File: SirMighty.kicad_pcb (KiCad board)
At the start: 2 copper layers, 61 x 20.5 mm, 49 parts, among them J1 Conn_01x20, J2 Conn_01x20, J3 USB_B_Micro, Q1 Q_DUAL_PMOS_S1G1D2S2G2D1, U2 AP7365-W-7, U4 AZ1117-5.0

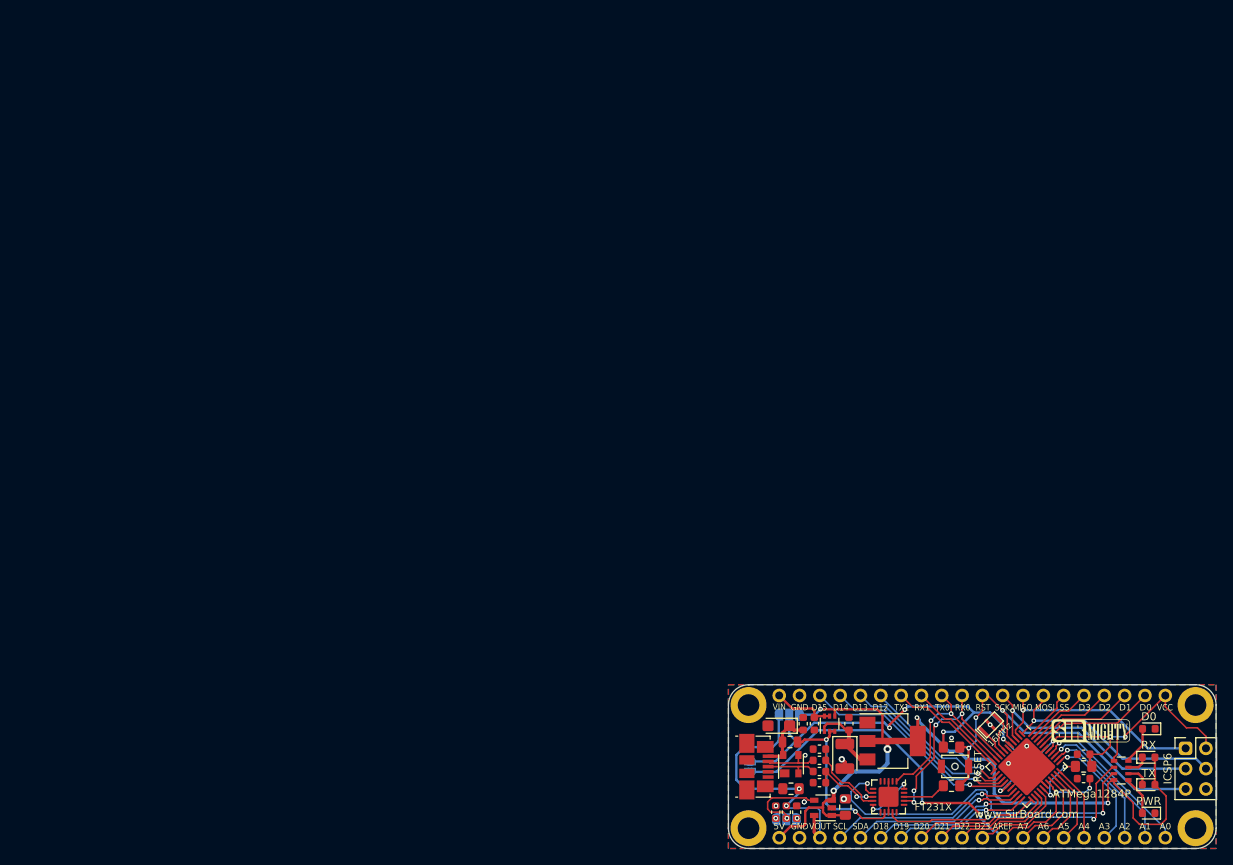
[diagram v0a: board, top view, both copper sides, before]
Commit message: Page Settings Updated
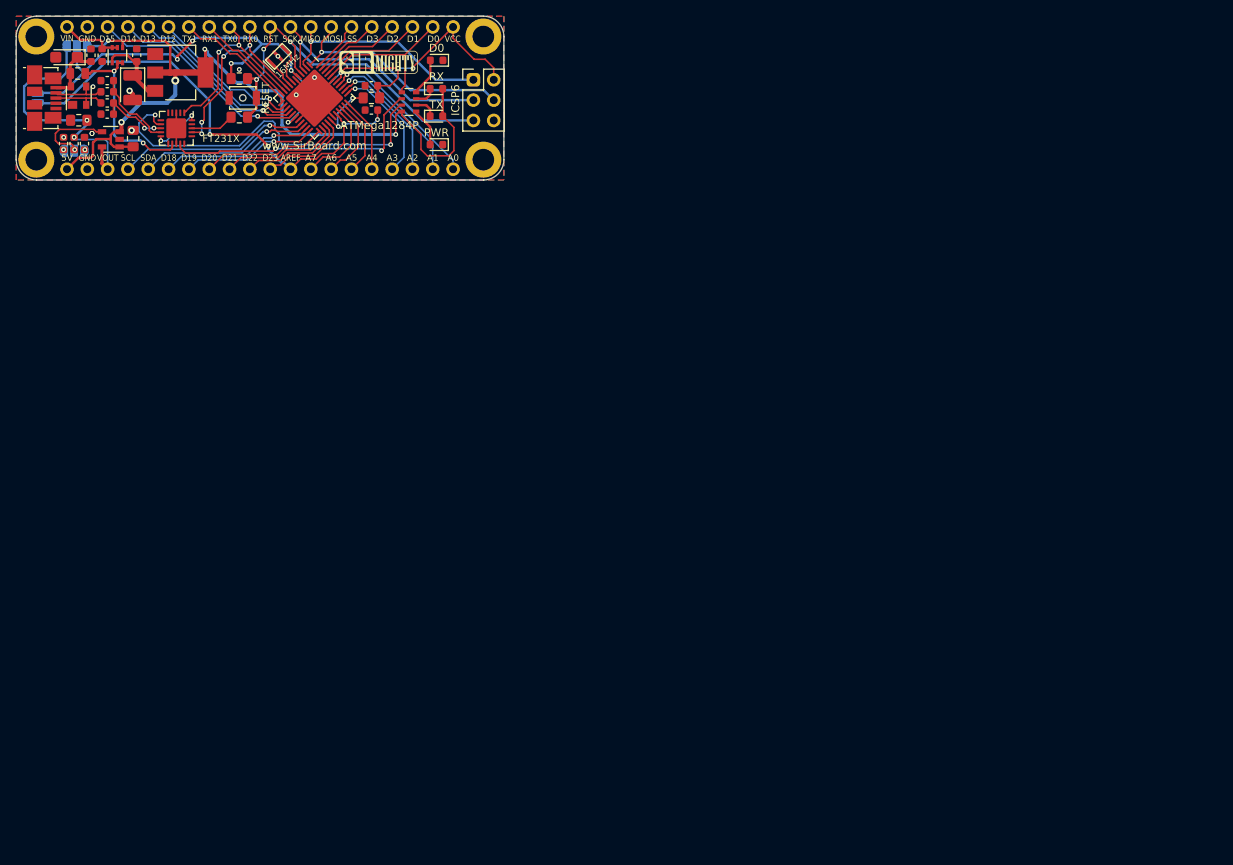
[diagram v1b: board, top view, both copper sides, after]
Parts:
- moved C10 122.1 mm to (48.6, 44.2)
- moved C11 122.1 mm to (68.7, 43.8)
- moved C5 122.1 mm to (55.9, 36.1)
- moved C6 122.1 mm to (50.2, 36.1)
- moved C8 122.1 mm to (47.1, 36.3)
- moved C9 122.1 mm to (55.4, 46.5)
- moved D1 122.1 mm to (48.6, 41.1)
- moved FT231X 122.1 mm to (60.8, 45.2)
- moved G*** 122.1 mm to (75.2, 41.4)
- moved G*** 122.1 mm to (51.3, 41.4)
- moved G*** 122.1 mm to (60.8, 41.4)
- moved G*** 122.1 mm to (86.1, 37.0)
- moved JP1 122.1 mm to (43.5, 41.4)
- moved JP3 122.1 mm to (48.4, 34.9)
- moved PWR 122.1 mm to (93.3, 47.2)
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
